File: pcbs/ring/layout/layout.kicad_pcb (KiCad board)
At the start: 2 copper layers, 56 x 6.2 mm, 60 parts, among them J1 ?, Q1 CSD13380F3T, Q2 CSD13380F3T, U1 BQ27427YZFR, U2 BQ29700, U3 nRF52833-QDAA, U4 MAX30102EFD+T, U5 LSM6DSOX, U6 ?, U7 TMP117AIDRVR, U8 TPS7A2018PDQN, Y1 8J32076001, Y2 3110M4-32.768DTTLLLL

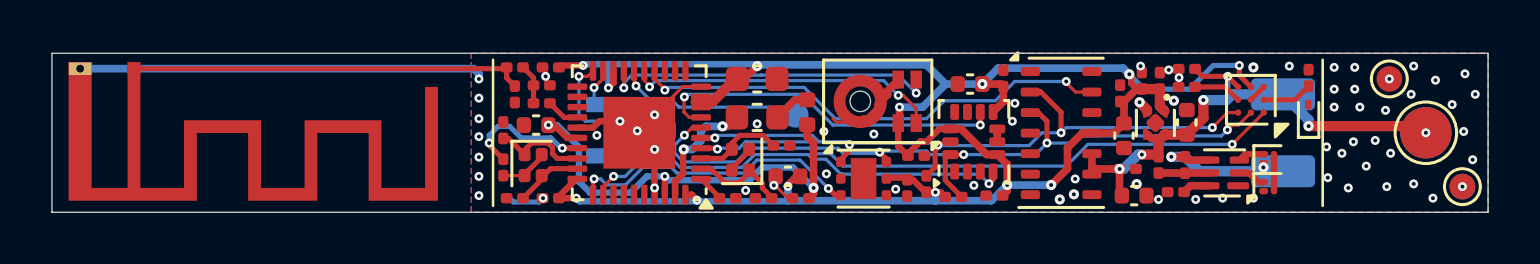
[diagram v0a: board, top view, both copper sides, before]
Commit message: reorganized for v2
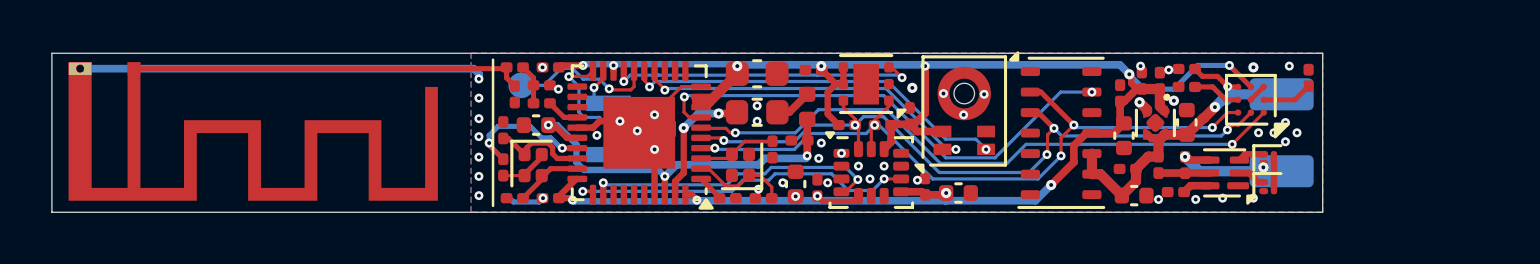
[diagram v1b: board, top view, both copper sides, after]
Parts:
- removed D1: ESD9B5.0ST5G, D_SOD-923:D_SOD-923
- removed TP2, TP5: , TestPoint_Pad_D2.0mm:TestPoint_Pad_D2.0mm
- removed TP3, TP4, TP6: , TestPoint_Pad_D1.0mm:TestPoint_Pad_D1.0mm
- moved TP1 10.8 mm to (136.6, 81.2)
- moved C22 6.91 mm to (148.1, 85.2), turned to 90 degrees
- moved C26 5.87 mm to (147.9, 80.7), turned to 180 degrees
- moved C23 5.21 mm to (152.3, 85.2)
- moved R1 5.01 mm to (149.2, 82.8)
- moved C24 4.27 mm to (153.6, 85.5), turned to 0 degrees
- moved U5 4.18 mm to (150.2, 84.7), turned to 0 degrees
- moved U7 3.69 mm to (150.0, 81.2), turned to 180 degrees
- moved MK1 3.40 mm to (153.8, 82.2), turned to 90 degrees
- moved R2 2.86 mm to (150.7, 82.8), turned to 180 degrees
- moved C15 2.25 mm to (147.4, 83.4)
- moved C25 1.57 mm to (151.7, 82.5), turned to 90 degrees
- moved C6 0.42 mm to (147.2, 85.1), turned to 90 degrees
- moved C11 0.38 mm to (146.3, 83.8), turned to -90 degrees
- moved L2 0.22 mm to (147.7, 82.1)
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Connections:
- U3 pad 14: hbt_int -> mic_data
- U3 pad 15: mic_data -> mic_clk
- U3 pad 17: mic_clk -> tmp_int
- U3 pad 31: tmp_int -> imu_int2
- U3 pad 4: sda -> scl
- U3 pad 5: scl -> sda
- U3 pad 7: imu_int2 -> hbt_int
- U7 pad 4: GND -> VDD
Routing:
- net VDD: track 81.8 -> 74.4 mm
- net VBATT: track 21.4 -> 14.1 mm, vias 6 -> 2
- net GND: track 35.7 -> 29.0 mm, vias 68 -> 46
- net imu_int1: track 17.1 -> 11.7 mm
- net cpu.dec4_6: track 18.2 -> 15.2 mm
- net bat_low: track 26.1 -> 24.1 mm
- net mic_clk: track 13.2 -> 15.0 mm
- net mic_data: track 12.2 -> 13.9 mm
- net rst: track 7.31 -> 5.69 mm
- net scl: track 26.9 -> 28.2 mm
- net battery.bat_vss: track 6.31 -> 5.24 mm
- net sda: track 27.2 -> 27.8 mm
- net tmp_int: track 11.5 -> 12.1 mm
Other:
- board size 56 x 6.2 mm -> 49.6 x 6.2 mm
